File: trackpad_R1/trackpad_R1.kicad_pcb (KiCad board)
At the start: 2 copper layers, 75.5 x 75 mm, 17 parts, among them J1 Conn_01x17

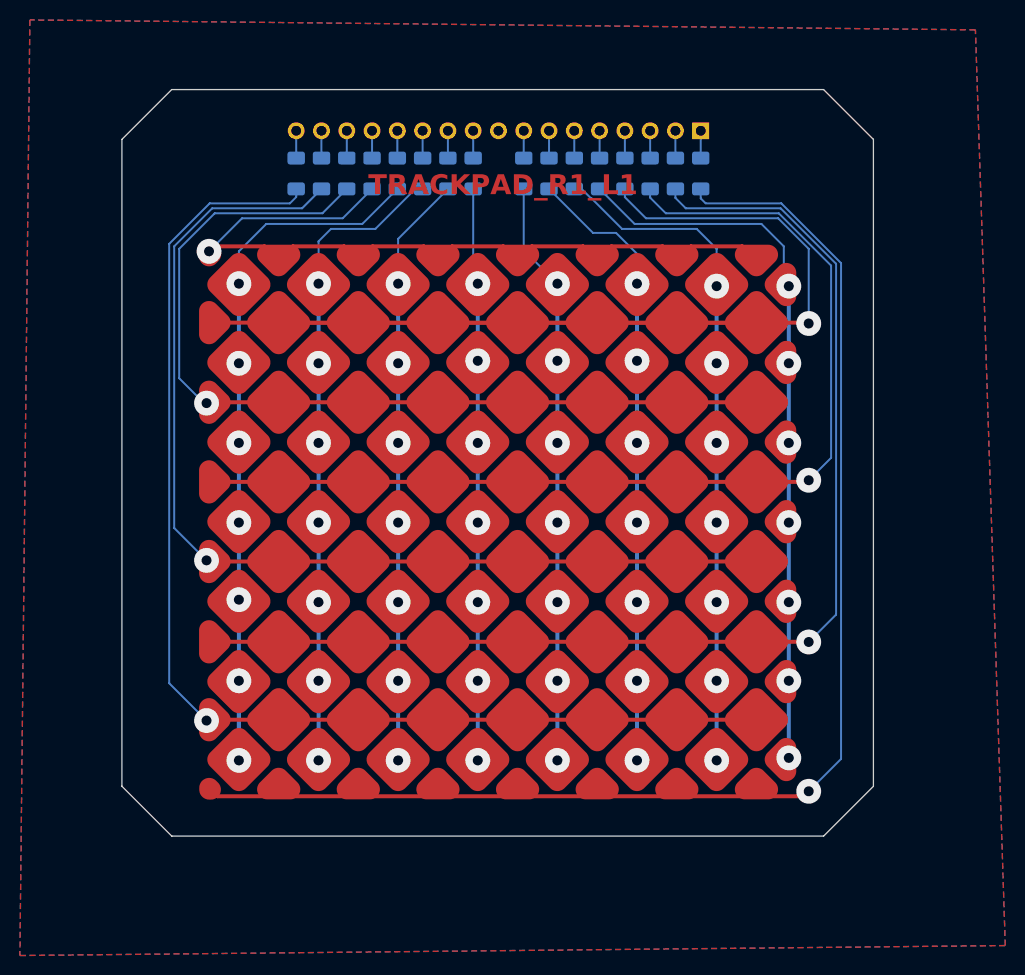
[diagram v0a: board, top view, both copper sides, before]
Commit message: progress
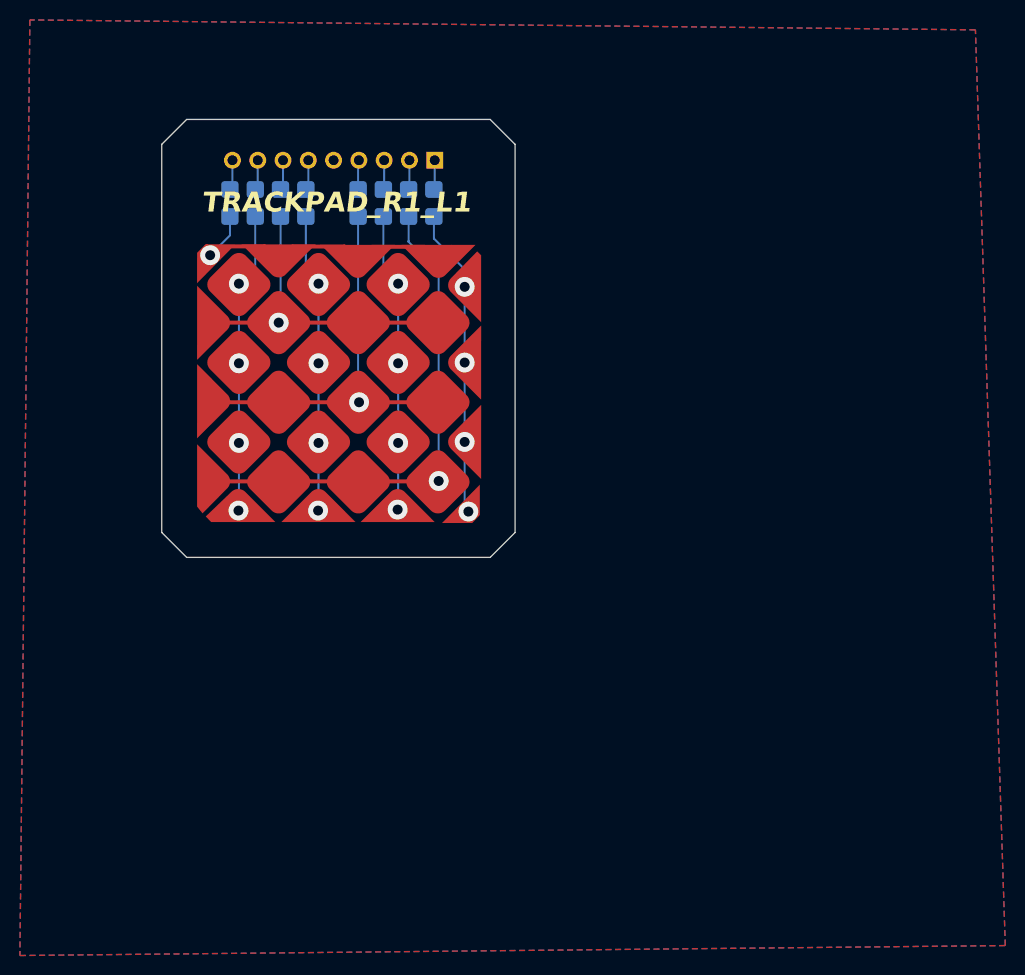
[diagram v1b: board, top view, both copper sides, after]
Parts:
- removed R10, R11, R12, R13, R14, R15, R16, R9: R, Resistor_SMD:R_1206_3216Metric_Pad1.30x1.75mm_HandSolder
- J1: value Conn_01x17 -> Conn_01x09; footprint Connector_PinHeader_2.54mm:PinHeader_1x17_P2.54mm_Horizontal -> Connector_PinHeader_2.54mm:PinHeader_1x09_P2.54mm_Horizontal
- R1, R2, R3, R4, R5, R6, R7: footprint Resistor_SMD:R_1206_3216Metric_Pad1.30x1.75mm_HandSolder -> Library:R_1206_3216Metric_Pad1.30x1.75mm_HandSolder_extra
- moved R8 29.7 mm to (52.1, 77.4)
- moved R6 29.7 mm to (57.2, 77.4)
- moved R5 29.7 mm to (59.7, 77.4)
- moved R7 29.7 mm to (54.6, 77.4)
- moved R1 27.0 mm to (72.6, 77.4)
- moved R4 27.0 mm to (65.0, 77.4)
- moved R2 27.0 mm to (70.1, 77.4)
- moved R3 27.0 mm to (67.5, 77.4)
- moved J1 26.9 mm to (72.7, 73.1)
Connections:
- J1 pad 5: Net-(J1-Pin_5) -> GND
- J1 pad 9: GND -> Net-(J1-Pin_9)
- R5 pad 1: Net-(J1-Pin_5) -> Net-(J1-Pin_6)
- R6 pad 1: Net-(J1-Pin_6) -> Net-(J1-Pin_7)
- R7 pad 1: Net-(J1-Pin_7) -> Net-(J1-Pin_8)
- R8 pad 1: Net-(J1-Pin_8) -> Net-(J1-Pin_9)
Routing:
- net unconnected-(R16-Pad2): track 118.6 -> 0.00 mm, vias 1 -> 0
- net unconnected-(R1-Pad2): track 140.2 -> 30.9 mm, vias 1 -> 4
- net unconnected-(R15-Pad2): track 103.7 -> 0.00 mm, vias 1 -> 0
- net unconnected-(R4-Pad2): track 137.0 -> 40.1 mm
- net unconnected-(R14-Pad2): track 91.0 -> 0.00 mm, vias 1 -> 0
- net unconnected-(R13-Pad2): track 82.9 -> 0.00 mm, vias 1 -> 0
- net unconnected-(R12-Pad2): track 77.8 -> 0.00 mm, vias 7 -> 0
- net unconnected-(R3-Pad2): track 105.5 -> 30.4 mm, vias 1 -> 4
- net unconnected-(R2-Pad2): track 120.9 -> 50.2 mm
- net unconnected-(R11-Pad2): track 64.9 -> 0.00 mm, vias 7 -> 0
- net unconnected-(R10-Pad2): track 59.6 -> 0.00 mm, vias 7 -> 0
- net unconnected-(R9-Pad2): track 57.7 -> 0.00 mm, vias 7 -> 0
- net unconnected-(R5-Pad2): track 72.3 -> 29.4 mm, vias 7 -> 4
- net unconnected-(R6-Pad2): track 68.3 -> 33.3 mm, vias 7 -> 1
- net unconnected-(R7-Pad2): track 62.5 -> 30.1 mm, vias 7 -> 4
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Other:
- board size 75.5 x 75 mm -> 35.5 x 44 mm
